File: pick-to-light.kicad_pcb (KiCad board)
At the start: 4 copper layers, 38.1 x 29.8 mm, 35 parts, among them IC1 ATMEGA168PA-A, P1 CONN_02X03, P2 CONN_02X03, Q1 BC849, Q2 BC849, SW1 SW_PUSH, SW2 SW_PUSH, U1 LD1117S33TR, Y1 Crystal

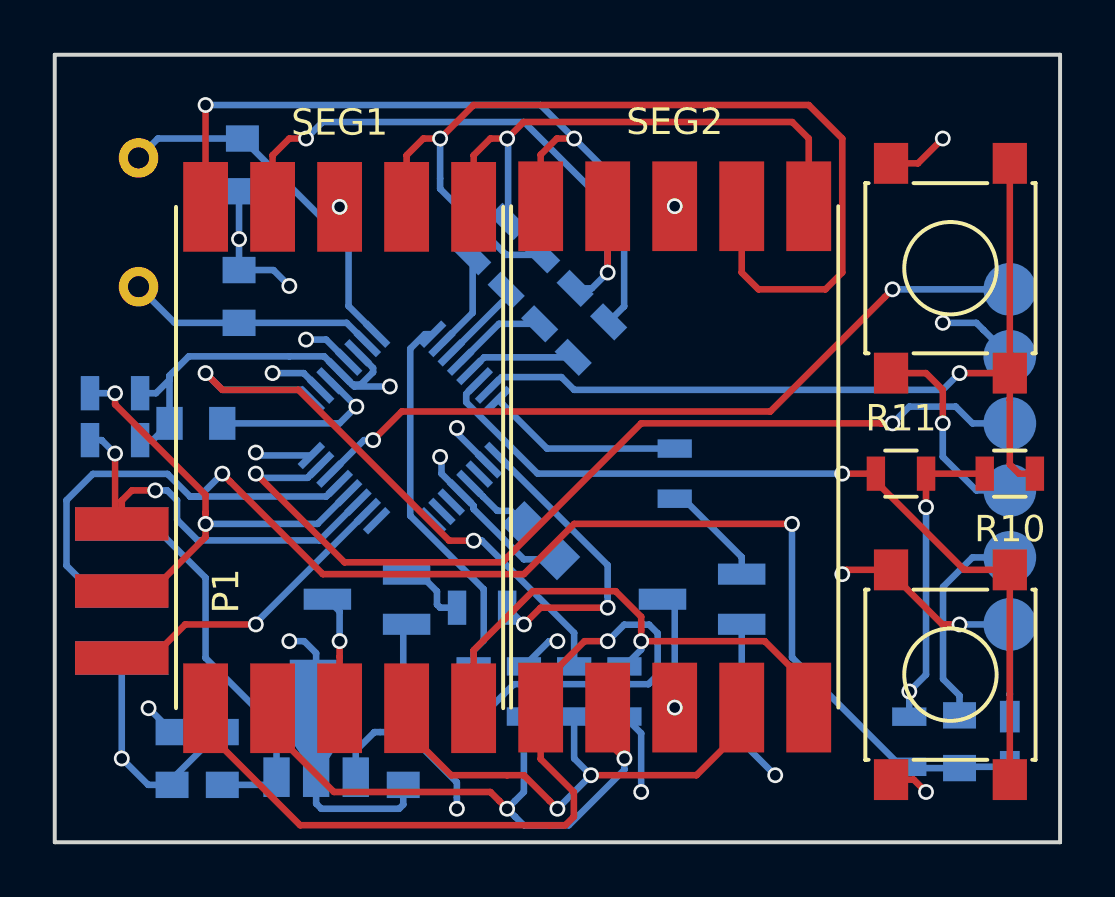
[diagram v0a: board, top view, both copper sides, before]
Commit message: Finished second round of layout.
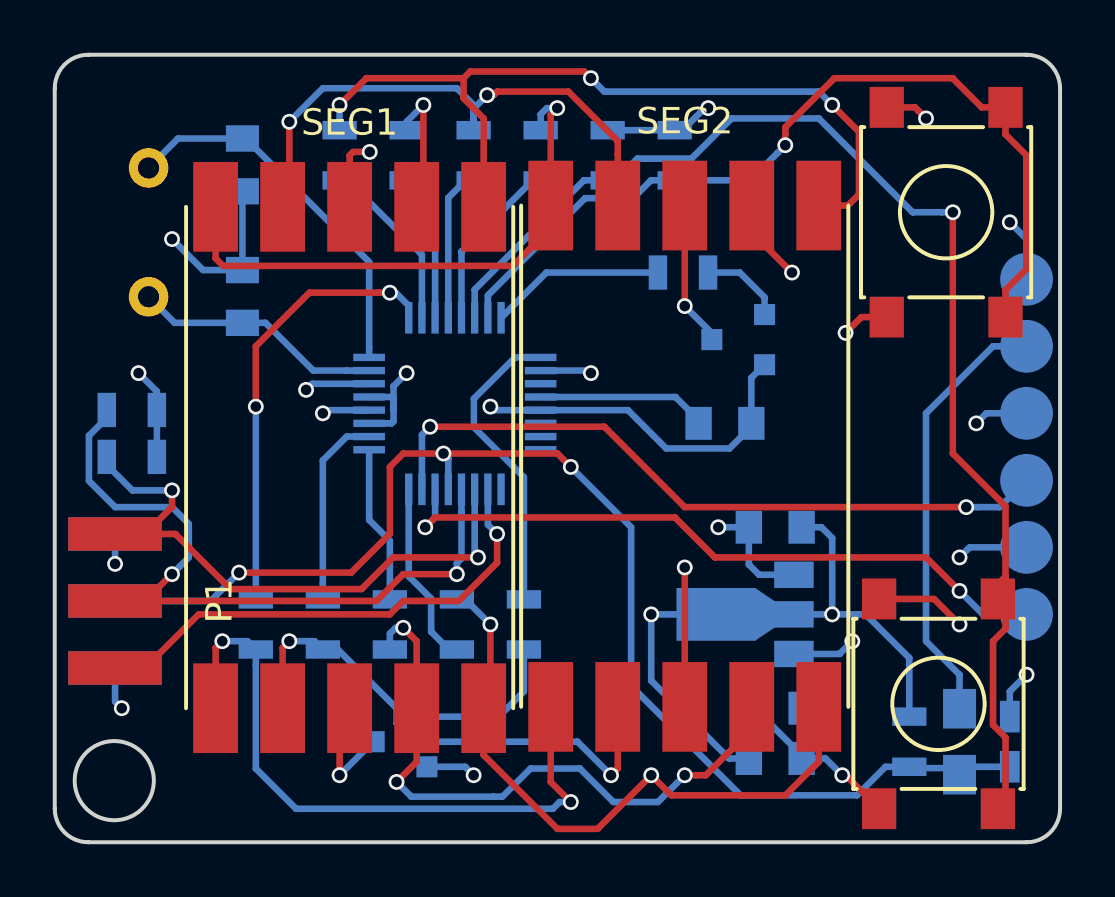
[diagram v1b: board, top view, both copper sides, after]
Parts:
- removed C1: 0.1uF, Capacitors_SMD:C_0805
- C6: footprint Capacitors_SMD:C_0805 -> Capacitors_SMD:C_0805_HandSoldering
- Q1, Q2: footprint TO_SOT_Packages_SMD:SOT-23_Handsoldering -> TO_SOT_Packages_SMD:SOT-23
- R10, R11: moved to B.Cu
- moved C4 22.9 mm to (133.3, 111.8), turned to 0 degrees
- moved C3 21.0 mm to (133.3, 109.9), turned to 180 degrees
- moved R10 17.5 mm to (129.5, 88.9), turned to 90 degrees
- moved U1 16.8 mm to (132.2, 106.3), turned to 270 degrees
- moved C5 16.6 mm to (133.3, 103.0), turned to 180 degrees
- moved R11 16.4 mm to (127.0, 88.9), turned to 90 degrees
- moved Q2 9.93 mm to (131.9, 95.9)
- moved R5 8.64 mm to (113.7, 106.7)
- moved C2 8.28 mm to (131.4, 99.1), turned to 0 degrees
- moved R6 8.03 mm to (116.2, 106.7)
- moved R12 7.63 mm to (129.9, 93.3), turned to 180 degrees
- moved R7 7.43 mm to (118.7, 106.7)
- moved R1 7.24 mm to (124.5, 88.9), turned to 270 degrees
- moved R8 6.84 mm to (121.3, 106.7)
- moved R4 6.54 mm to (116.8, 88.9), turned to 270 degrees
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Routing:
- net RAW: track 14.9 -> 37.3 mm, vias 0 -> 2
- net Net-(IC1-Pad32): track 25.7 -> 7.00 mm, vias 2 -> 0
- net Net-(IC1-Pad1): track 23.7 -> 6.00 mm, vias 2 -> 0
- net GND: track 69.5 -> 52.2 mm
- net Net-(IC1-Pad14): track 32.4 -> 48.3 mm
- net Net-(IC1-Pad2): track 20.2 -> 7.39 mm, vias 2 -> 0
- net Net-(R3-Pad1): track 38.5 -> 25.7 mm, vias 1 -> 2
- net Net-(R5-Pad1): track 36.7 -> 25.2 mm, vias 1 -> 2
- net A5: track 17.8 -> 28.8 mm
- net Net-(Q1-Pad3): track 21.3 -> 31.8 mm
- net Net-(R4-Pad1): track 21.2 -> 31.4 mm, vias 1 -> 3
- net Net-(C6-Pad2): track 8.12 -> 16.8 mm
- net TX0: track 35.4 -> 26.8 mm
- net Net-(R1-Pad1): track 29.8 -> 21.3 mm, vias 2 -> 1
- net A4: track 15.7 -> 24.1 mm
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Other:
- outline, holes or cut-outs redrawn
- rule trace_min: 0.2 -> 0.007874
- rule via_min_size: 0.4 -> 0.015748
